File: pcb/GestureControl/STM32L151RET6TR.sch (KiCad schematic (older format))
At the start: 33 parts, among them J10 EXTERN I2C, J11 Conn_01x02, J12 Conn_01x02, J17 Conn_01x01, J18 Conn_01x01, J19 Conn_01x01, J7 FTDI, J8 Conn_01x06, J9 UART, U6 STM32L151RETx, U7 STM32F401RETx, Y1 8MHz, Y2 32kHz

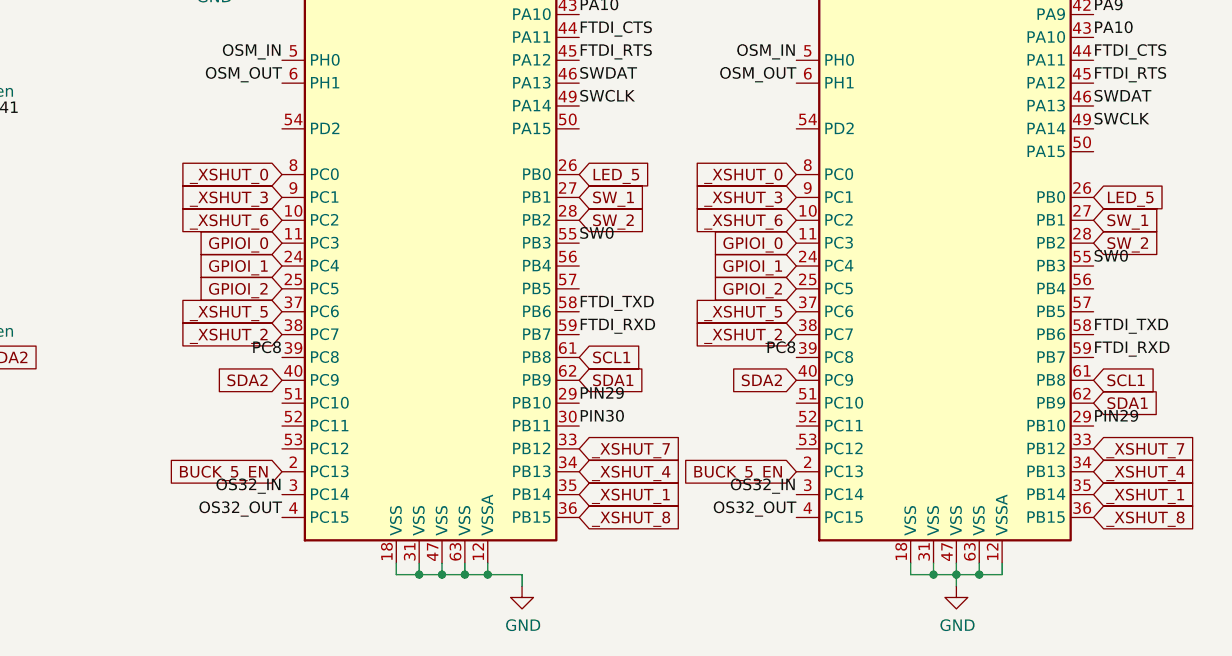
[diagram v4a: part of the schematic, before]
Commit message: add PCB V12
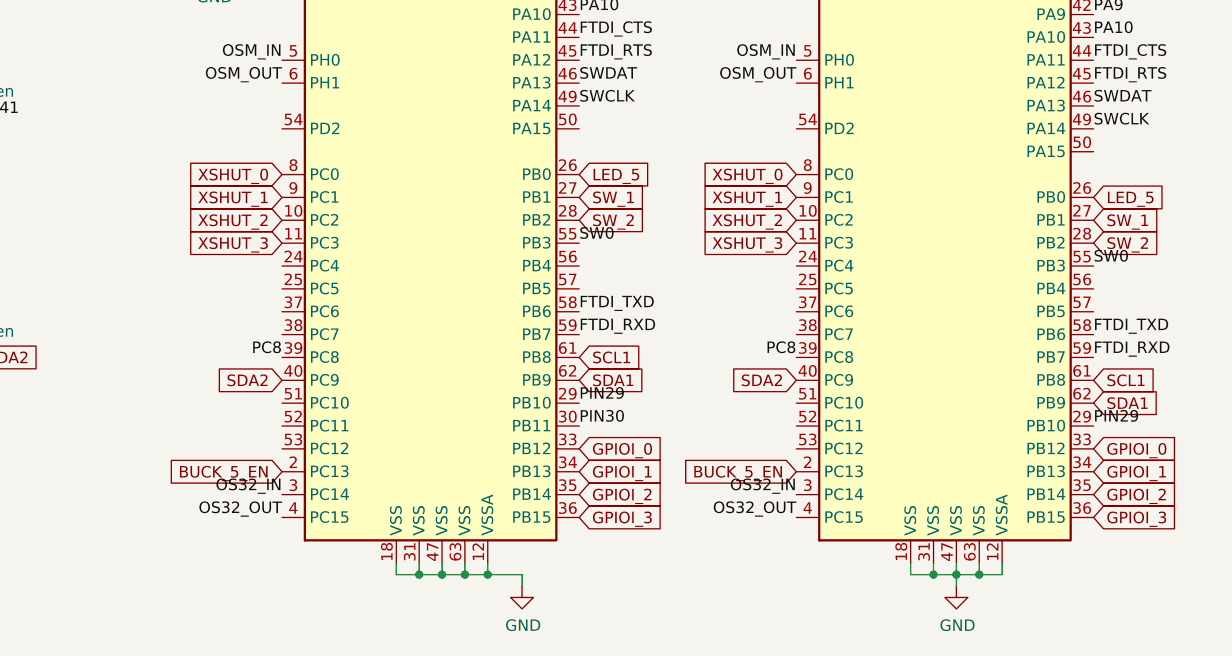
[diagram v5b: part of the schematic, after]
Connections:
- net _XSHUT_1 is gone; now on net GPIOI_2: U6.35 (PB14), U7.35 (PB14)
- net _XSHUT_4 is gone; now on net GPIOI_1: U6.34 (PB13), U7.34 (PB13)
- net _XSHUT_7 is gone; now on net GPIOI_0: U6.33 (PB12), U7.33 (PB12)
- net GPIOI_0: no longer U6.11 (PC3), U7.11 (PC3)
- net GPIOI_1: no longer U6.24 (PC4), U7.24 (PC4)
- net GPIOI_2: no longer U6.25 (PC5), U7.25 (PC5)
- net _XSHUT_0 renamed XSHUT_0
- net _XSHUT_2: no longer names the net of U6.38 (PC7)
- net _XSHUT_2: no longer U7.38 (PC7)
- net _XSHUT_3 renamed XSHUT_1
- net _XSHUT_5: no longer names the net of U6.37 (PC6)
- net _XSHUT_5: no longer U7.37 (PC6)
- net _XSHUT_6 renamed XSHUT_2
- net _XSHUT_8 renamed GPIOI_3
- new net XSHUT_3: U6.11 (PC3), U7.11 (PC3)
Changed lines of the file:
@@
 $Descr A3 16535 11693
 encoding utf-8
-Sheet 5 5
+Sheet 3 3
 Title ""
 Date ""
@@
 LED_4
 Text GLabel 4650 4550 0    50   Input ~ 0
-_XSHUT_0
-Text GLabel 4650 4650 0    50   Input ~ 0
-_XSHUT_3
-Text GLabel 4650 4750 0    50   Input ~ 0
-_XSHUT_6
-Text GLabel 4650 4850 0    50   Input ~ 0
+XSHUT_0
+Text GLabel 5950 5750 2    50   Input ~ 0
 GPIOI_0
-Text GLabel 4650 4950 0    50   Input ~ 0
+Text GLabel 5950 5850 2    50   Input ~ 0
 GPIOI_1
-Text GLabel 4650 5050 0    50   Input ~ 0
+Text GLabel 5950 5950 2    50   Input ~ 0
 GPIOI_2
 Wire Wire Line
@@
 Text Label 6900 4150 2    50   ~ 0
 OSM_OUT
-Text GLabel 6900 4550 0    50   Input ~ 0
-_XSHUT_0
-Text GLabel 6900 4650 0    50   Input ~ 0
-_XSHUT_3
-Text GLabel 6900 4750 0    50   Input ~ 0
-_XSHUT_6
-Text GLabel 6900 4850 0    50   Input ~ 0
-GPIOI_0
-Text GLabel 6900 4950 0    50   Input ~ 0
-GPIOI_1
-Text GLabel 6900 5050 0    50   Input ~ 0
-GPIOI_2
 Text GLabel 8200 5550 2    50   Input ~ 0
 SDA1
@@
 Text Label 2900 4300 2    50   ~ 0
 PIN29
-Text GLabel 8200 5950 2    50   Input ~ 0
-_XSHUT_1
-Text GLabel 8200 5850 2    50   Input ~ 0
-_XSHUT_4
-Text GLabel 8200 5750 2    50   Input ~ 0
-_XSHUT_7
-Text GLabel 5950 5950 2    50   Input ~ 0
-_XSHUT_1
-Text GLabel 5950 5850 2    50   Input ~ 0
-_XSHUT_4
-Text GLabel 5950 5750 2    50   Input ~ 0
-_XSHUT_7
-Text GLabel 5950 6050 2    50   Input ~ 0
-_XSHUT_8
-Text GLabel 4650 5250 0    50   Input ~ 0
-_XSHUT_2
-Text GLabel 4650 5150 0    50   Input ~ 0
-_XSHUT_5
-Text GLabel 8200 6050 2    50   Input ~ 0
-_XSHUT_8
-Text GLabel 6900 5150 0    50   Input ~ 0
-_XSHUT_5
-Text GLabel 6900 5250 0    50   Input ~ 0
-_XSHUT_2
 Text GLabel 6900 5850 0    50   Input ~ 0
 BUCK_5_EN
@@
 	-1   0    0    1
 $EndComp
+Text GLabel 5950 6050 2    50   Input ~ 0
+GPIOI_3
+Text GLabel 8200 5750 2    50   Input ~ 0
+GPIOI_0
+Text GLabel 8200 5850 2    50   Input ~ 0
+GPIOI_1
+Text GLabel 8200 5950 2    50   Input ~ 0
+GPIOI_2
+Text GLabel 8200 6050 2    50   Input ~ 0
+GPIOI_3
+Text GLabel 4650 4650 0    50   Input ~ 0
+XSHUT_1
+Text GLabel 4650 4750 0    50   Input ~ 0
+XSHUT_2
+Text GLabel 4650 4850 0    50   Input ~ 0
+XSHUT_3
+Text GLabel 6900 4550 0    50   Input ~ 0
+XSHUT_0
+Text GLabel 6900 4650 0    50   Input ~ 0
+XSHUT_1
+Text GLabel 6900 4750 0    50   Input ~ 0
+XSHUT_2
+Text GLabel 6900 4850 0    50   Input ~ 0
+XSHUT_3
 $EndSCHEMATC

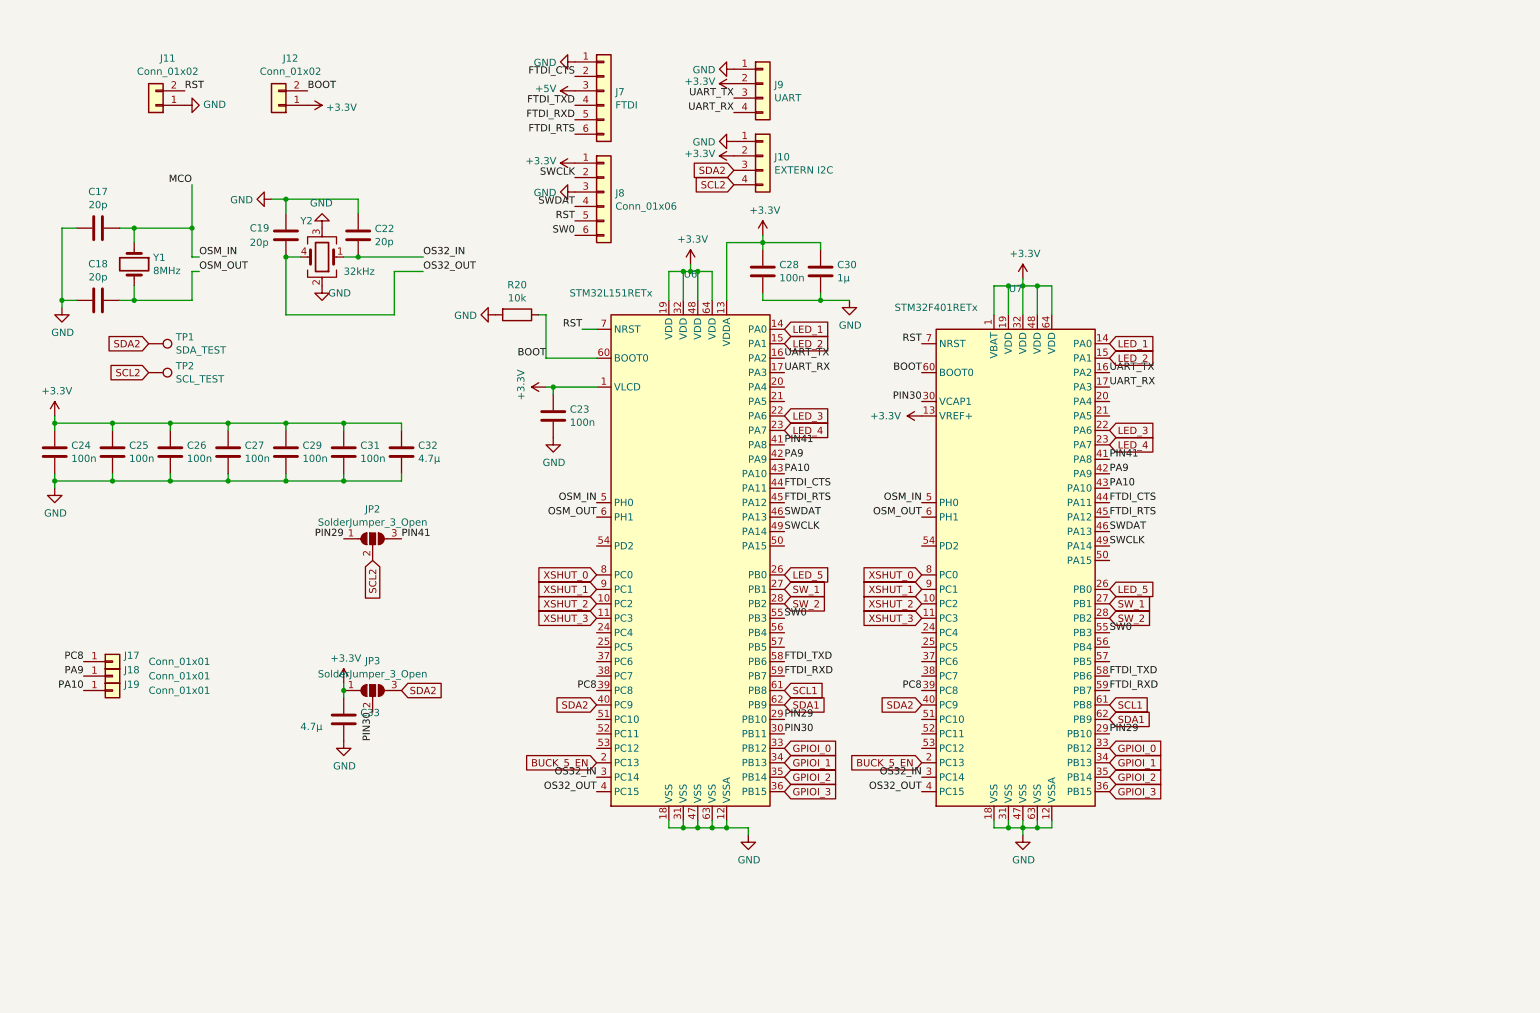
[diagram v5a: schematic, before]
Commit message: cleanup PCB V0.1
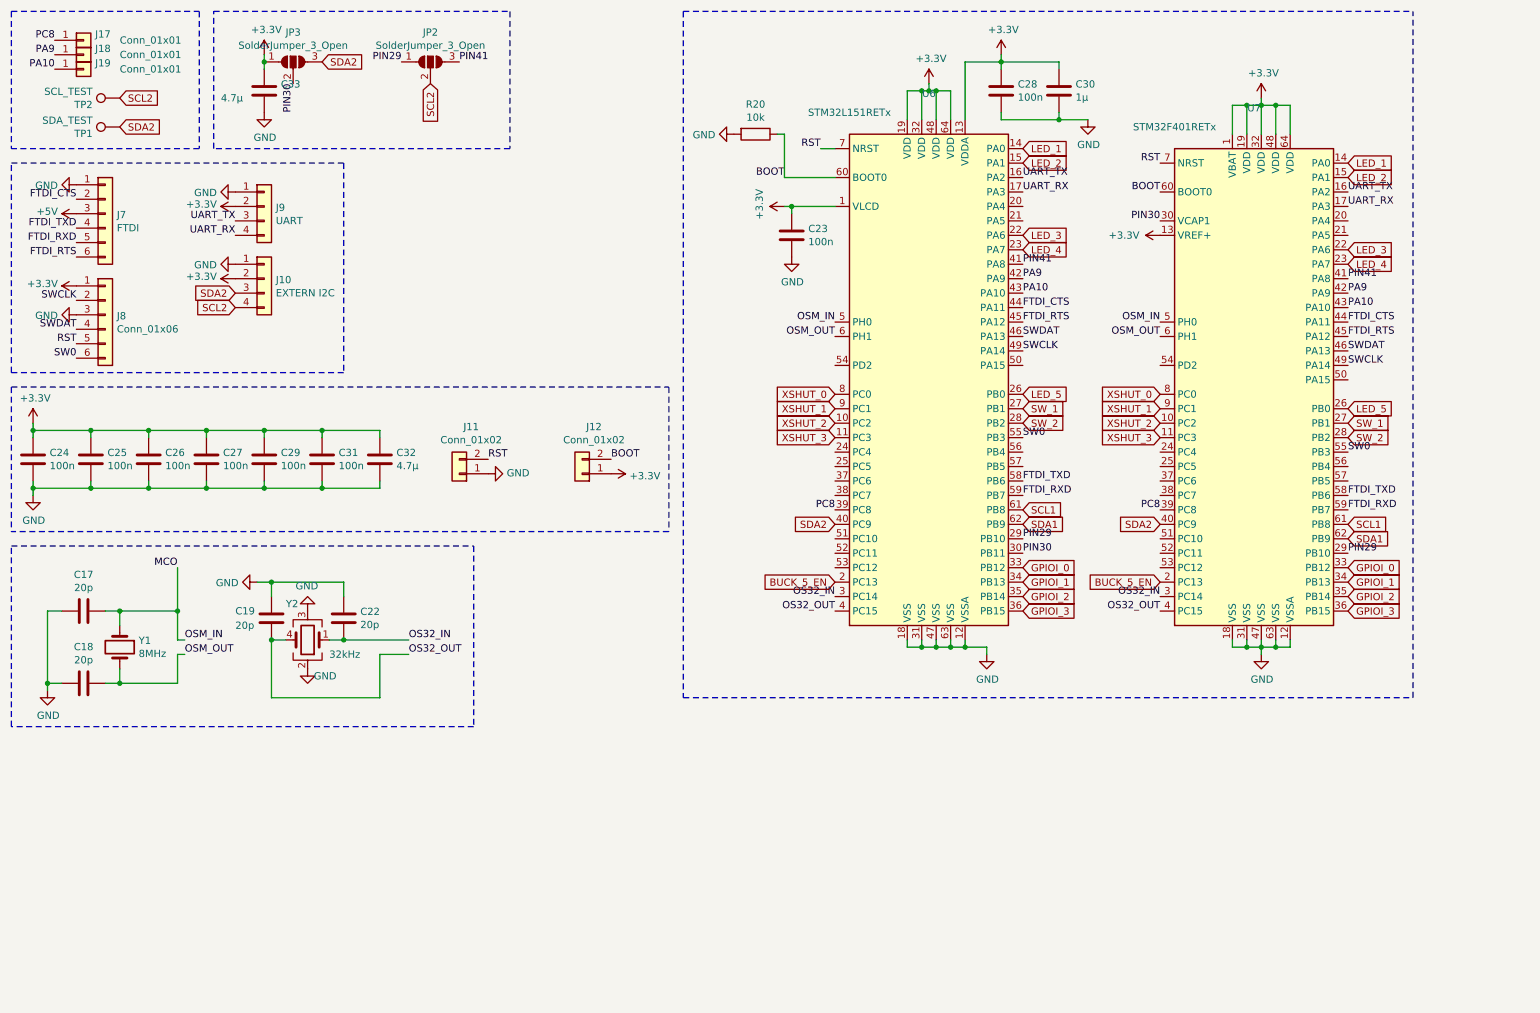
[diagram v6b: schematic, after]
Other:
- moved on the sheet: C17, C18, C19, C22, C23, C24, C25, C26, C27, C28, C29, C30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
